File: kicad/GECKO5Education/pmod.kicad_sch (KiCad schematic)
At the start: 24 parts, among them J3 Conn_02x06_Odd_Even, J4 Conn_02x06_Odd_Even, J6 Conn_01x08_Socket, U13 NCP1529A, U14 NCP1529A, U6 LFE5U-85F-6BG381x, U8 LP5907MFX-2.5, X1 ECS-2520MV-500-BL-TR

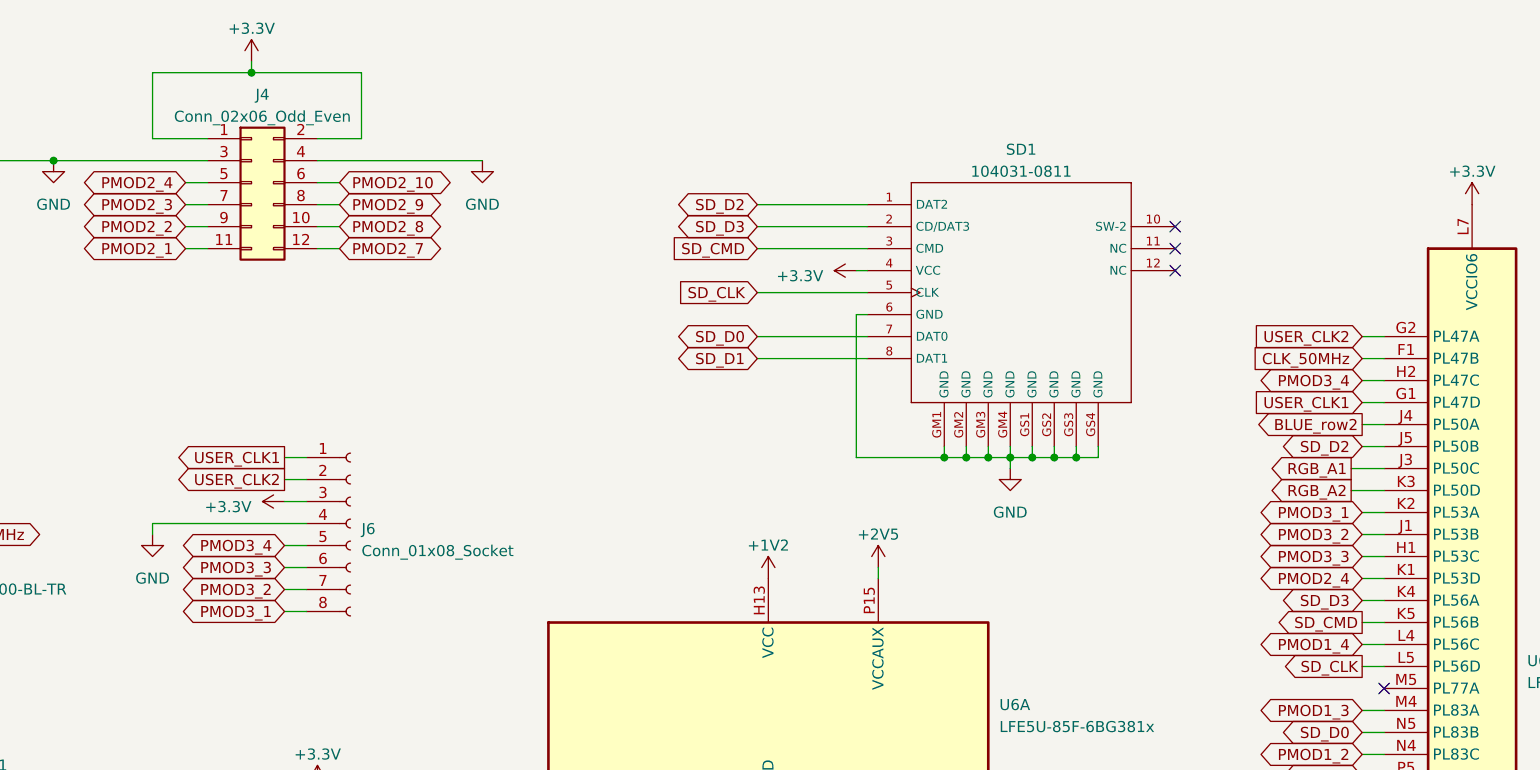
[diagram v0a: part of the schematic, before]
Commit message: Small modifications plus added documentation
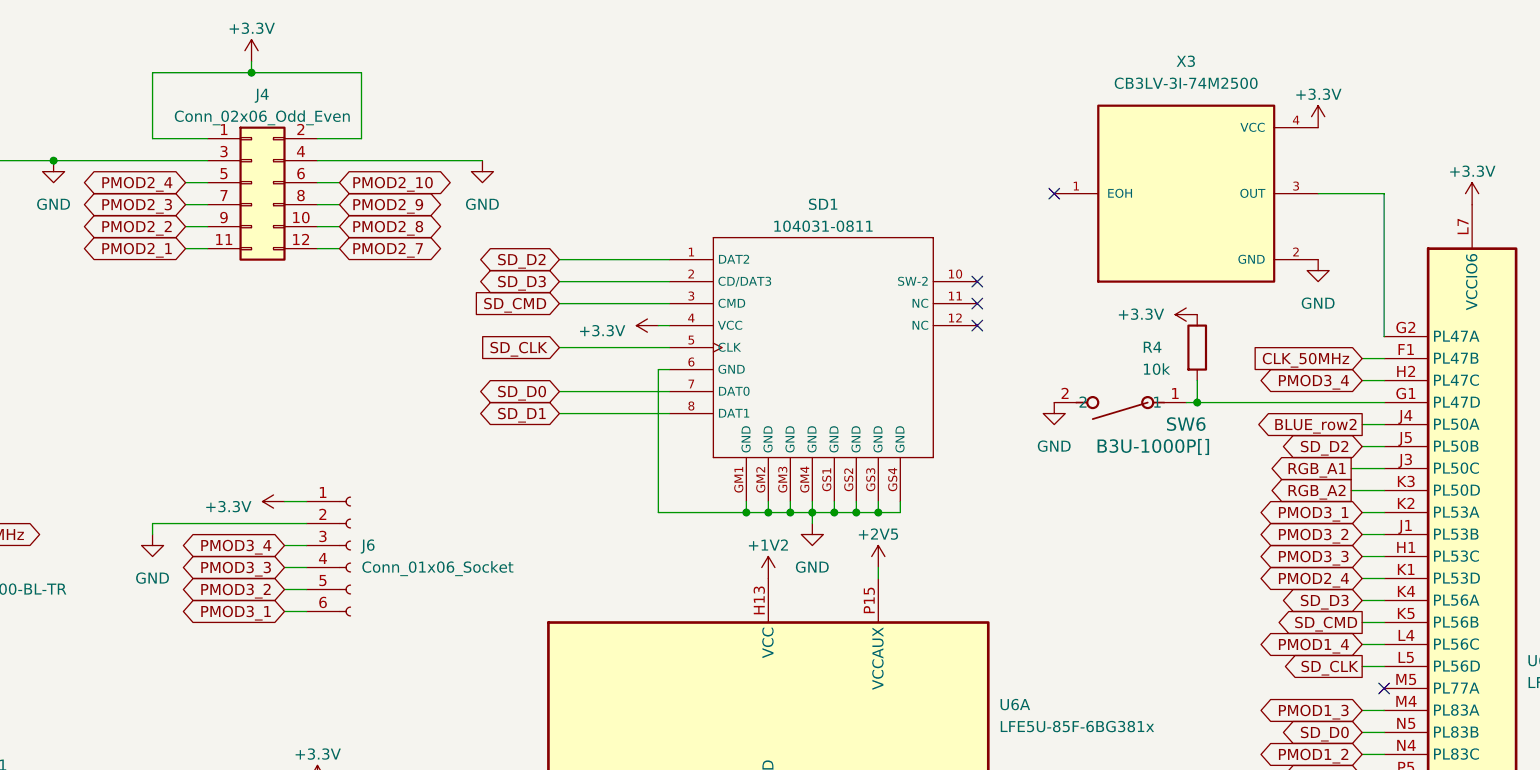
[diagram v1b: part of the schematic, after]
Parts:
- removed J6: Conn_01x08_Socket, Connector_PinSocket_2.54mm:PinSocket_1x08_P2.54mm_Horizontal, symbol Connector:Conn_01x08_Socket
- added J6: Conn_01x06_Socket, Connector_PinSocket_2.54mm:PinSocket_1x06_P2.54mm_Horizontal, symbol Connector:Conn_01x06_Socket
- added R4: 10k, Resistor_SMD:R_0402_1005Metric, symbol Device:R
- added SW6: B3U-1000P[], gecko4education:SW_B3U-1000P_OMR, symbol gecko5education:B3U-1000P[]
- added X3: CB3LV-3I-74M2500, gecko4education:OSCCC700X500X180-4N, symbol gecko5education:CB3LV-3I-74M2500
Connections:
- net +3.3V: now also J6.1 (Pin_1), R4.1, X3.4 (VCC)
- net GND: now also J6.2 (Pin_2), SW6.2, X3.2 (GND)
- net PMOD3_1: now also J6.6 (Pin_6)
- net PMOD3_2: now also J6.5 (Pin_5)
- net PMOD3_3: now also J6.4 (Pin_4)
- net PMOD3_4: now also J6.3 (Pin_3)
- net USER_CLK1: no longer names the net of U6.G1 (PL47D)
- net USER_CLK1: now also R4.2, SW6.1
- net USER_CLK2: no longer names the net of U6.G2 (PL47A)
- net USER_CLK2: now also X3.3 (OUT)
- no-connect marks 4 -> 5
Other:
- moved on the sheet: SD1
